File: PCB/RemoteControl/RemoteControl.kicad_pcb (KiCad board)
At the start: 2 copper layers, 86.4 x 56.6 mm, 12 parts, among them J1 USB_C_Receptacle_USB2.0_14P, J2 Conn_01x05_Socket, J3 Conn_01x05_Pin, J4 Conn_01x04_Socket, J5 Conn_01x06_Socket, U1 STM32L031K6Tx, U2 TC1262-33

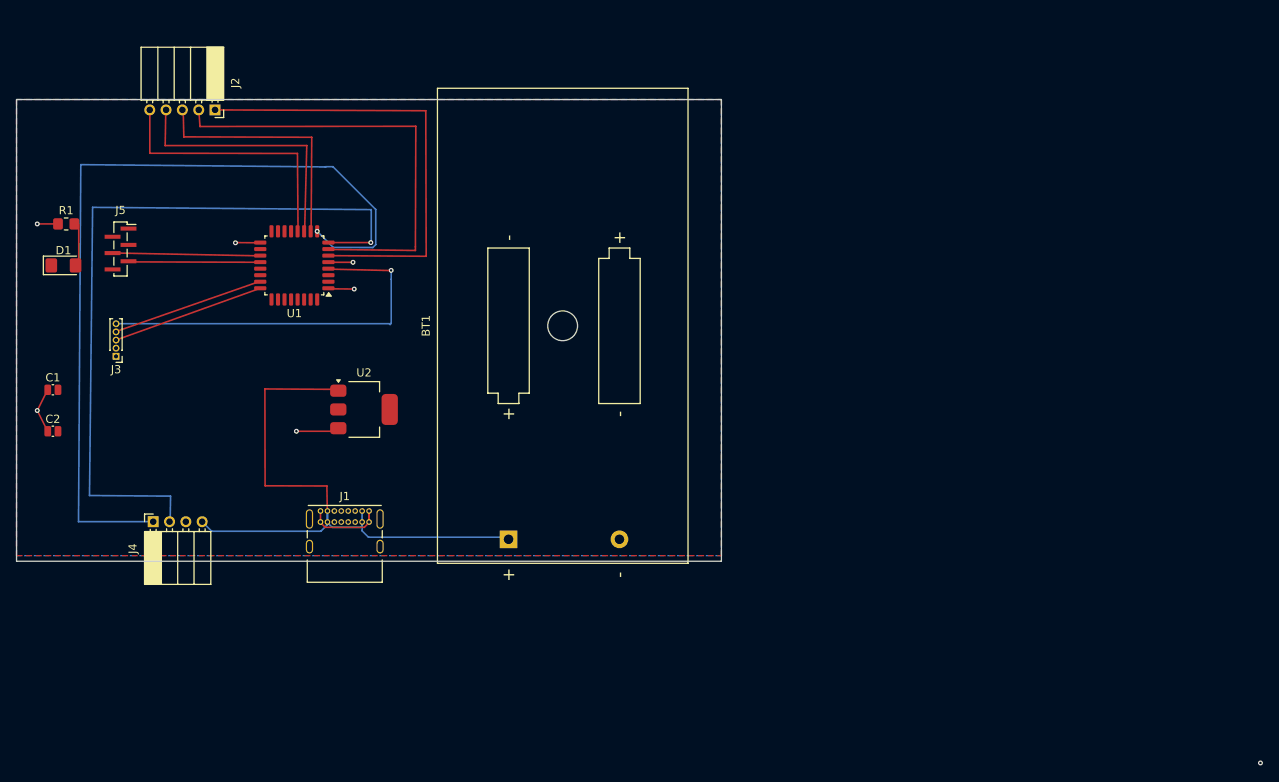
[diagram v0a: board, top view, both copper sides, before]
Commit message: Pushing
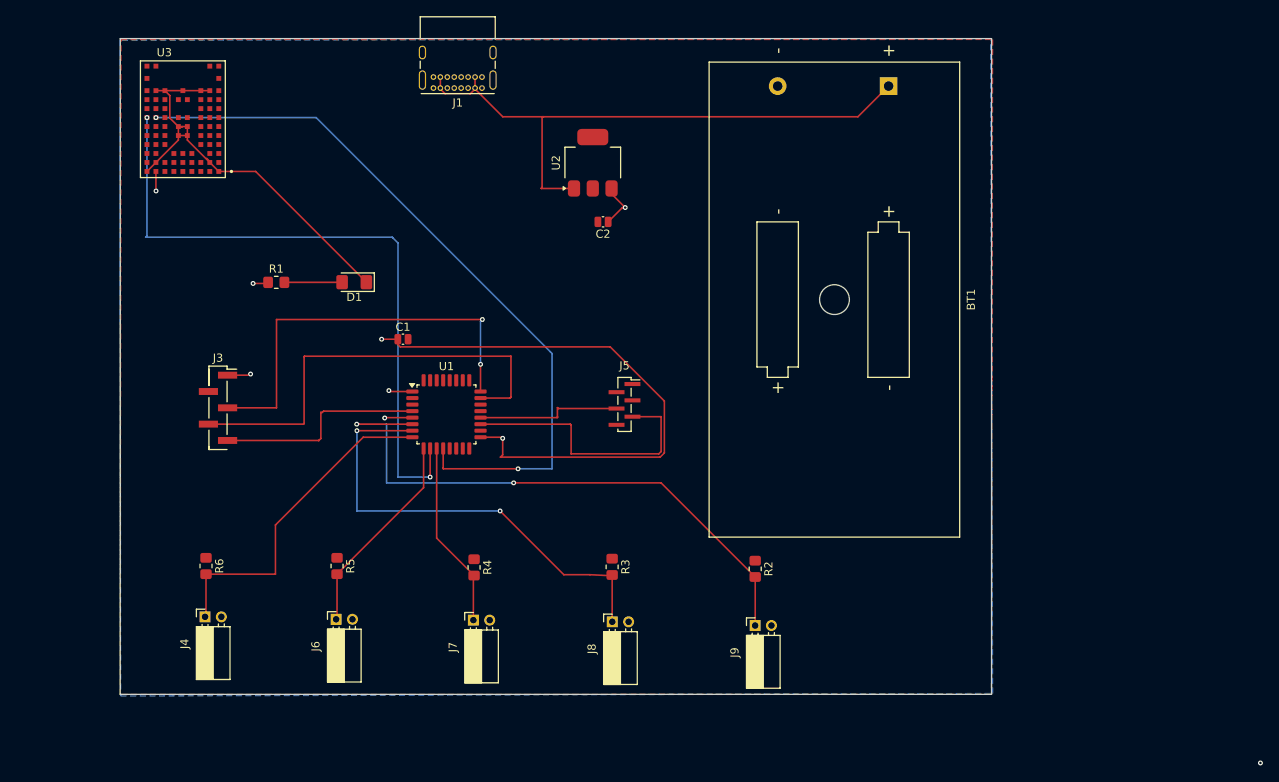
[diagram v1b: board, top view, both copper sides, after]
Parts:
- removed J2: Conn_01x05_Socket, Connector_PinSocket_2.00mm:PinSocket_1x05_P2.00mm_Horizontal
- added J6: Conn_01x02_Socket, Connector_PinSocket_2.00mm:PinSocket_1x02_P2.00mm_Horizontal, F.Cu at (95.0, 119.6)
- added J7: Conn_01x02_Socket, Connector_PinSocket_2.00mm:PinSocket_1x02_P2.00mm_Horizontal, F.Cu at (111.9, 119.7)
- added J8: Conn_01x02_Socket, Connector_PinSocket_2.00mm:PinSocket_1x02_P2.00mm_Horizontal, F.Cu at (128.9, 119.9)
- added J9: Conn_01x02_Socket, Connector_PinSocket_2.00mm:PinSocket_1x02_P2.00mm_Horizontal, F.Cu at (146.4, 120.3)
- added R2: R, Resistor_SMD:R_0805_2012Metric_Pad1.20x1.40mm_HandSolder, F.Cu at (146.4, 113.4)
- added R3: R, Resistor_SMD:R_0805_2012Metric_Pad1.20x1.40mm_HandSolder, F.Cu at (128.9, 113.1)
- added R4: R, Resistor_SMD:R_0805_2012Metric_Pad1.20x1.40mm_HandSolder, F.Cu at (111.9, 113.2)
- added R5: R, Resistor_SMD:R_0805_2012Metric_Pad1.20x1.40mm_HandSolder, F.Cu at (95.1, 113.0)
- added R6: R, Resistor_SMD:R_0805_2012Metric_Pad1.20x1.40mm_HandSolder, F.Cu at (79.1, 113.0)
- added U3: NORA-W106-00B, NORA-W106-00B:XCVR_NORA-W106-00B, F.Cu at (76.3, 58.3)
- J3: footprint Connector_PinHeader_1.00mm:PinHeader_1x05_P1.00mm_Vertical -> Connector_PinHeader_2.00mm:PinHeader_1x05_P2.00mm_Vertical_SMD_Pin1Right
- J4: value Conn_01x04_Socket -> Conn_01x02_Socket; footprint Connector_PinSocket_2.00mm:PinSocket_1x04_P2.00mm_Horizontal -> Connector_PinSocket_2.00mm:PinSocket_1x02_P2.00mm_Horizontal
- moved BT1 72.5 mm to (162.7, 54.2), turned to -90 degrees
- moved C2 72.1 mm to (127.7, 70.9), turned to 180 degrees
- moved J5 64.6 mm to (130.4, 93.2)
- moved J1 55.5 mm to (112.9, 54.5), turned to 180 degrees
- moved C1 43.3 mm to (103.2, 85.2)
- moved U2 41.2 mm to (126.5, 63.6), turned to 90 degrees
- moved D1 35.7 mm to (97.3, 78.3), turned to 180 degrees
- moved R1 26.7 mm to (87.7, 78.3)
- moved U1 26.1 mm to (108.6, 94.5), turned to 0 degrees
- moved J3 14.0 mm to (80.6, 93.6), turned to 0 degrees
- moved J4 13.3 mm to (79.0, 119.3)
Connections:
- J4 pad 1: RX -> Finger5
- J4 pad 2: TX -> +3.3V
- U1 pad 10: Finger3 -> RX
- U1 pad 11: Finger4 -> Finger3
- U1 pad 12: Finger5 -> TX
- U1 pad 19: debug_tx -> debug_rx
- U1 pad 20: debug_rx -> debug_tx
- U1 pad 8: TX -> Finger5
- U1 pad 9: RX -> Finger4
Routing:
- net +3.3V: track 0.00 -> 89.9 mm, vias 6 -> 8
- net TX: track 5.25 -> 90.5 mm, vias 1 -> 2
- net Finger1: track 0.00 -> 73.8 mm, vias 0 -> 2
- net RX: track 20.8 -> 82.1 mm, vias 1 -> 2
- net Finger2: track 0.00 -> 54.4 mm, vias 0 -> 2
- net SWDIO: track 0.00 -> 54.1 mm
- net SWSCLK: track 0.00 -> 50.9 mm, vias 0 -> 2
- net gnd: track 10.6 -> 52.5 mm
- net Finger5: track 0.00 -> 41.0 mm
- net debug_rx: track 0.00 -> 33.6 mm
- net +5V: track 45.1 -> 74.3 mm
- net Finger4: track 0.00 -> 25.4 mm
- net Finger3: track 0.00 -> 23.0 mm
- net debug_tx: track 0.00 -> 17.9 mm
- net NRST: track 40.3 -> 26.0 mm, vias 1 -> 0
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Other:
- board size 86.4 x 56.6 mm -> 106.8 x 80.3 mm
